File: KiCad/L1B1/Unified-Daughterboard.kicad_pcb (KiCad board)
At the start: 2 copper layers, 18 x 16.5 mm, 14 parts, among them J1 TYPE-C-31-M12_13, J2 SM04B-SRSS-TB(LF)(SN), U1 TPD4E05U06DQAR

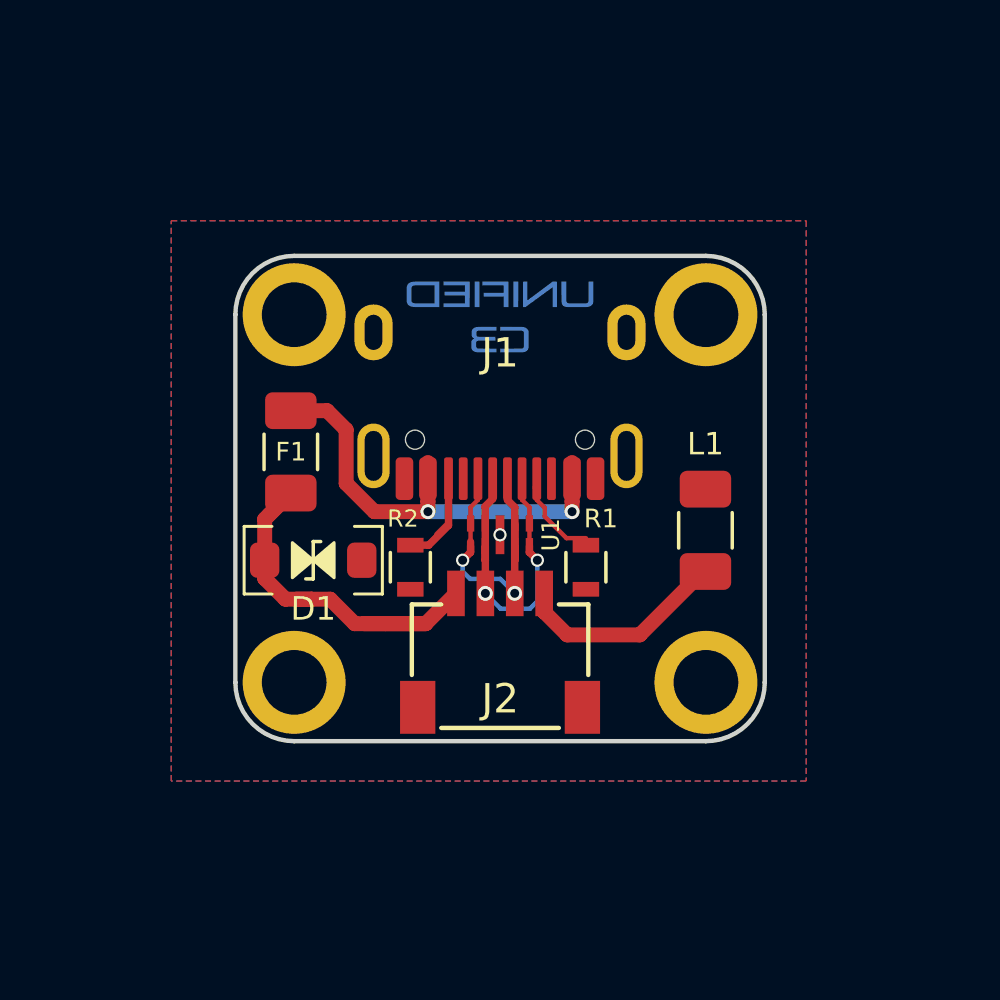
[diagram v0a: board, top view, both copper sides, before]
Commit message: Make the db
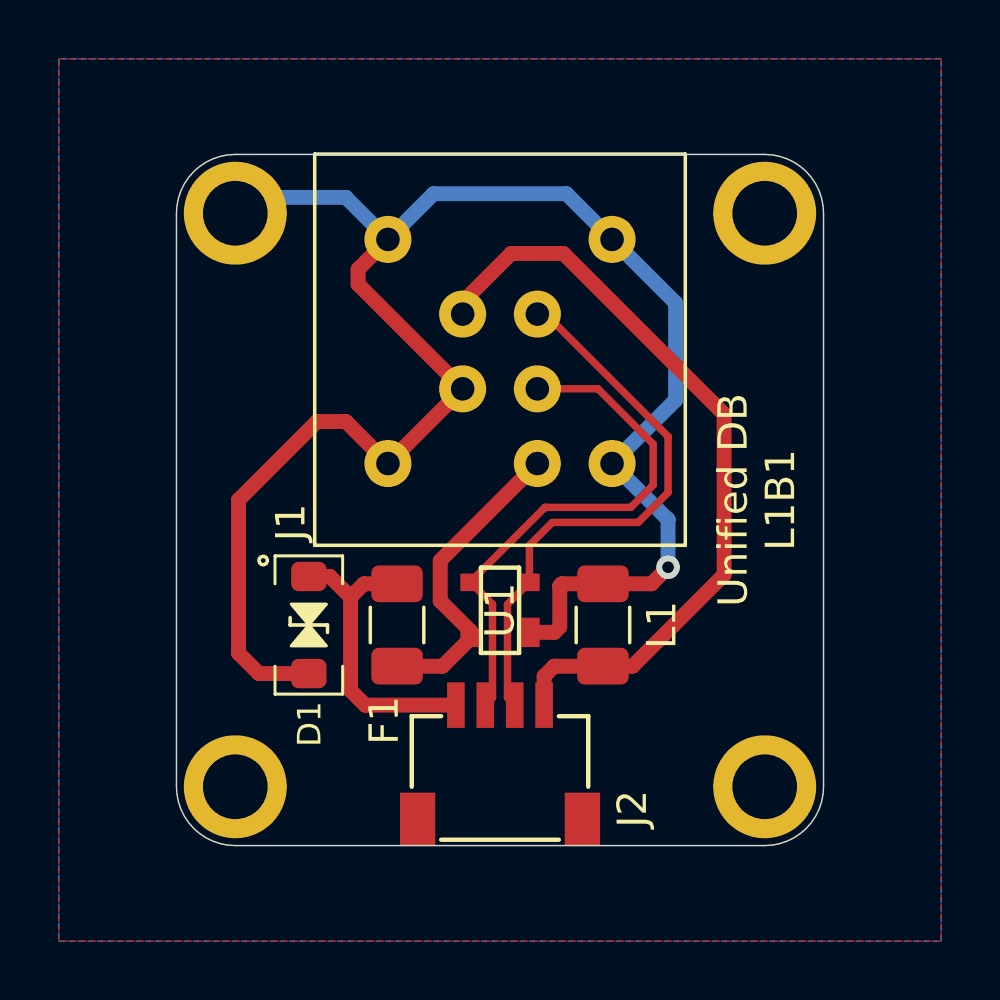
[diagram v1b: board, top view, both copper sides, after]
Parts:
- removed G1: Unified-Daughterboard-Logo, Unified-Daughterboard-Logo:Unified-Daughterboard-Logo.pretty
- removed G2: Unified-Daughterboard-Name, Unified-Daughterboard-Logo:Unified-Daughterboard-Name.pretty
- removed R1, R2: 5.1k, Resistors_SMD:R_0603
- J1: value TYPE-C-31-M12_13 -> EXG.1B.305.HLN; footprint acheron_Connectors:TYPE-C-31-M-12 -> locallib:EXG.1B.305.HLN
- U1: value TPD4E05U06DQAR -> PRTR5V0U2X; footprint acheron_Components:USON-10_2.5x1.0mm_P0.5mm -> random-keyboard-parts:SOT143B
- moved MH3 22.6 mm to (84.0, 55.1)
- moved MH2 16.4 mm to (66.0, 55.1)
- moved MH1 16.2 mm to (66.0, 74.6)
- moved F1 6.91 mm to (71.5, 69.1), turned to 90 degrees
- moved J1 5.05 mm to (75.0, 59.8), turned to 0 degrees
- moved L1 4.74 mm to (78.5, 69.1)
- moved MH4 4.07 mm to (84.0, 74.6)
- moved J2 3.80 mm to (75.0, 76.6)
- moved U1 2.57 mm to (75.0, 68.6), turned to 180 degrees
- moved D1 2.21 mm to (68.5, 69.1), turned to 90 degrees
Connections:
- J2 pad 2: DA- -> DN
- J2 pad 3: DA+ -> DP
- U1 pad 1: DA+ -> GNDPWR
- U1 pad 2: DA- -> DP
- U1 pad 3: GNDPWR -> DN
- U1 pad 4: DA+ -> VBUS
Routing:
- net GNDPWR: track 0.14 -> 60.3 mm
- net DP: track 0.00 -> 19.4 mm
- net GND: track 7.36 -> 26.2 mm
- net DN: track 0.00 -> 18.3 mm
- net DA+: track 13.6 -> 0.00 mm, vias 2 -> 0
- net DA-: track 13.4 -> 0.00 mm, vias 2 -> 0
- net Net-(J1-PadB5): track 6.33 -> 0.00 mm
- net VBUS: track 15.4 -> 10.6 mm, vias 2 -> 0
- net VCC: track 14.7 -> 10.4 mm
- net Net-(J1-PadA5): track 3.84 -> 0.00 mm
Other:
- board size 18 x 16.5 mm -> 22 x 23.5 mm
- board text added: "Unified DB L1B1"
